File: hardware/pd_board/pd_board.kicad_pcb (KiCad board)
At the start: 2 copper layers, 48.4 x 35.6 mm, 48 parts, among them J1 USB_C_Receptacle_USB2.0_16P, J2 CC1_TP, J3 CC2_TP, J4 Debug Port, J5 UART_Port, J6 VBUS_JP, J7 VCONN_JP, J8 VIN_ENA_JP, U1 FUSB302BMPX, U2 TPS5420D, U3 STM32F072CBUx

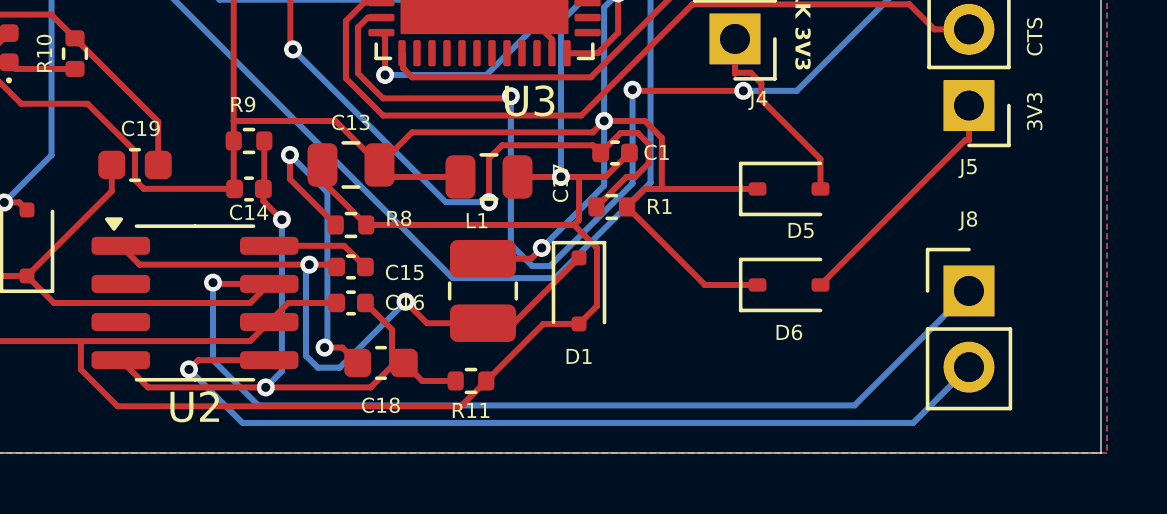
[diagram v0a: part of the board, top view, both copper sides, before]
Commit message: update
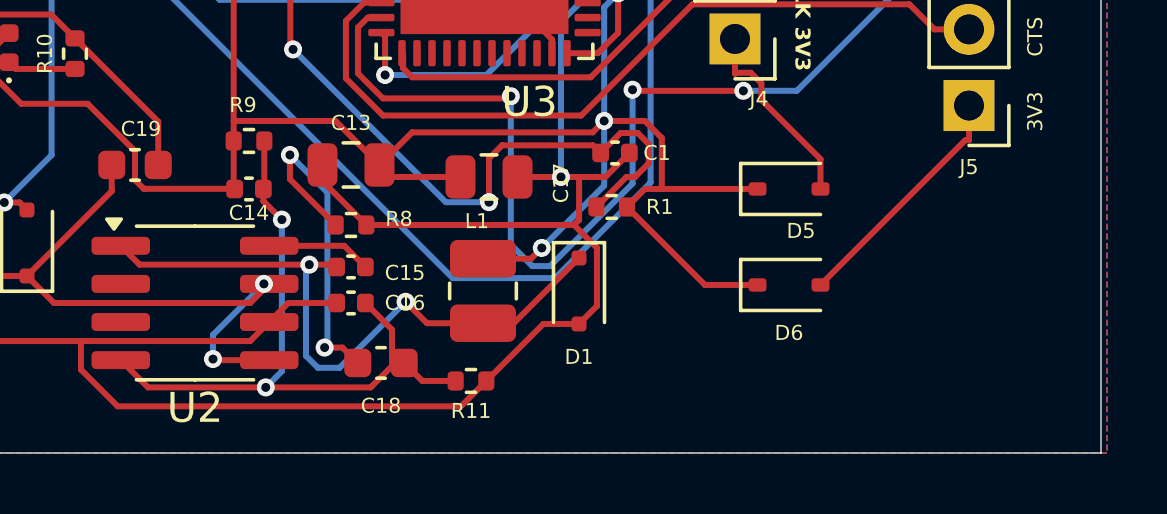
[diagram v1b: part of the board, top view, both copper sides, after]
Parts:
- removed J8: VIN_ENA_JP, Connector_PinHeader_2.54mm:PinHeader_1x02_P2.54mm_Vertical
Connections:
- C19 pad 1: /VIN -> Net-(D3-K)
- D3 pad 1: /VIN -> Net-(D3-K)
- D4 pad 1: /VIN -> Net-(D3-K)
- U2 pad 5: /VIN_ENA -> Net-(D3-K)
- U2 pad 7: /VIN -> Net-(D3-K)
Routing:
- net /VIN: track 48.9 -> 0.00 mm, vias 1 -> 0
- net /VIN_ENA: track 30.3 -> 0.00 mm, vias 1 -> 0
- net Net-(D3-K): track 0.00 -> 22.1 mm, vias 0 -> 2

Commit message: update
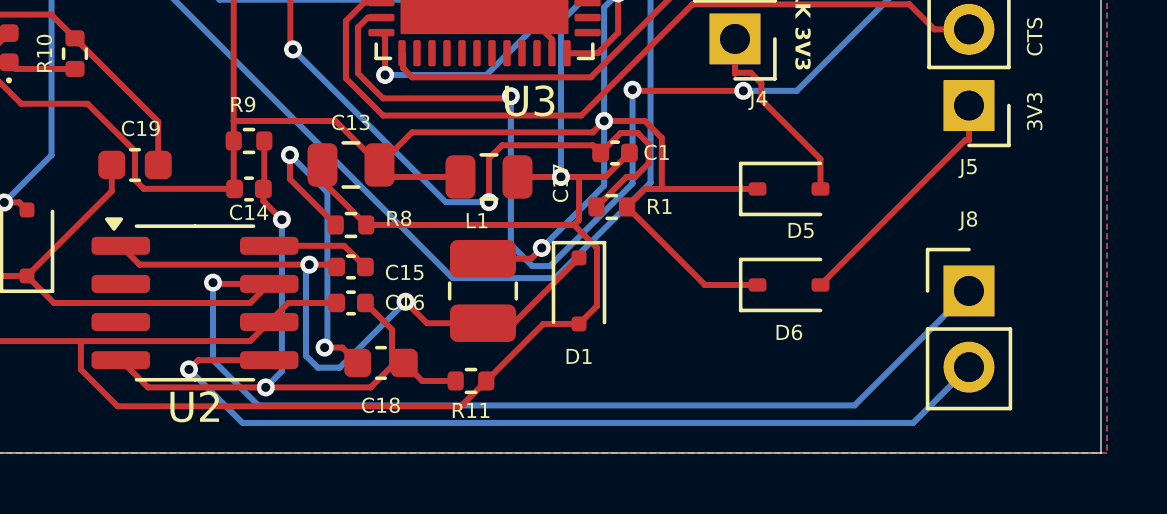
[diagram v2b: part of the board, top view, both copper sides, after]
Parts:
- added J8: VIN_ENA_JP, Connector_PinHeader_2.54mm:PinHeader_1x02_P2.54mm_Vertical, F.Cu at (149.6, 104.2)
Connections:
- C19 pad 1: Net-(D3-K) -> /VIN
- D3 pad 1: Net-(D3-K) -> /VIN
- D4 pad 1: Net-(D3-K) -> /VIN
- U2 pad 5: Net-(D3-K) -> /VIN_ENA
- U2 pad 7: Net-(D3-K) -> /VIN
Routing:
- net /VIN: track 0.00 -> 48.9 mm, vias 0 -> 1
- net /VIN_ENA: track 0.00 -> 30.3 mm, vias 0 -> 1
- net Net-(D3-K): track 22.1 -> 0.00 mm, vias 2 -> 0
